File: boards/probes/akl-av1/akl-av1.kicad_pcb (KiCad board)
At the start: 4 copper layers, 23.8 x 10.5 mm, 35 parts, among them J1 U.FL, J2 TIPRES, J3 TIPRES, J4 SMPM, U1 LTC1983-5, U2 ADP7142ACPZN-R7, U3 ADP7182_DFN8, U4 BUF802

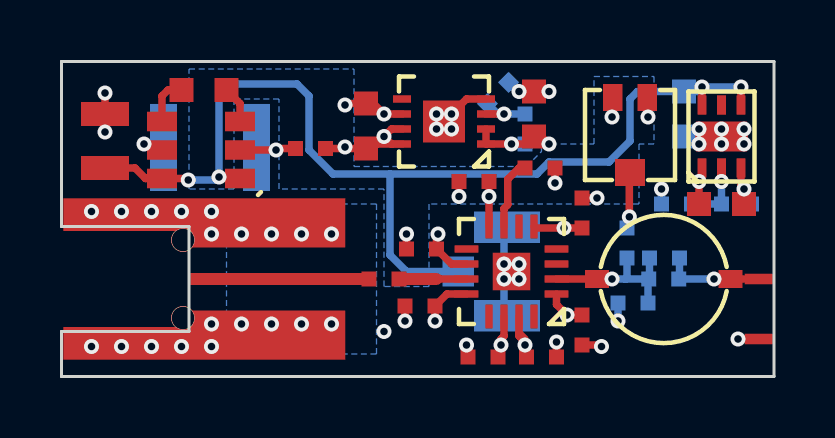
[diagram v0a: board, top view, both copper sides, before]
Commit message: Updated AKL-AV1 design files for v0.3 prototype
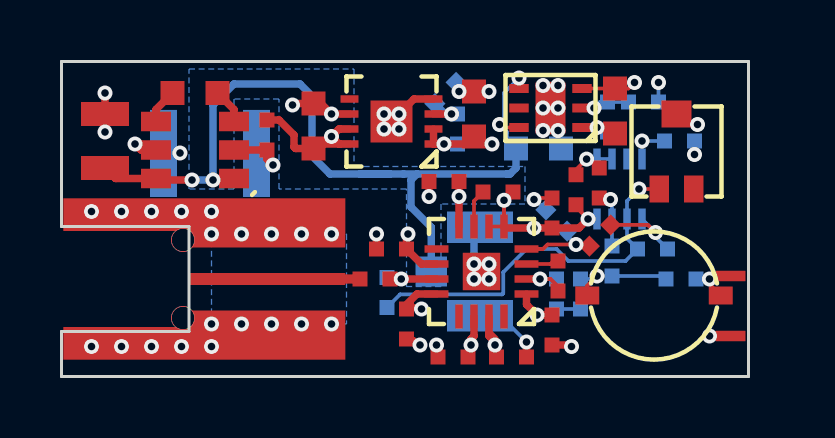
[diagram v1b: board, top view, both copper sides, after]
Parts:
- added C17: 0.47 uF, azonenberg_pcb:EIA_0402_CAP_NOSILK, F.Cu at (64.4, 48.0)
- added C18: 56 pF, azonenberg_pcb:EIA_0402_CAP_NOSILK, B.Cu at (67.0, 50.0)
- added C19: 330 pF, azonenberg_pcb:EIA_0402_CAP_NOSILK, B.Cu at (63.8, 51.5)
- added C20: 100 pF, azonenberg_pcb:EIA_0402_CAP_NOSILK, B.Cu at (63.8, 49.0)
- added R12: 80.6K, azonenberg_pcb:EIA_0402_RES_NOSILK, B.Cu at (58.1, 51.5)
- added R13: 2K, azonenberg_pcb:EIA_0402_RES_NOSILK, F.Cu at (65.2, 49.5)
- added R14: 10M, azonenberg_pcb:EIA_0402_RES_NOSILK, F.Cu at (63.8, 50.9)
- added R9: 3312J-1-203E, azonenberg_pcb:RES_TRIM_BOURNS_3312, F.Cu at (67.8, 46.8)
- added U5: ADA4075-2, azonenberg_pcb:DFN_8_0.5MM_2x2MM_NOPAD, B.Cu at (65.8, 48.0)
- C16: value 800 fF -> 0.47 uF
- R11: value 3312J-1-103E1 -> 30; footprint azonenberg_pcb:RES_TRIM_BOURNS_3312 -> azonenberg_pcb:EIA_0402_RES_NOSILK; moved to B.Cu
- R6: value 1M -> 806K
- R7: value 1M -> 200K; footprint azonenberg_pcb:EIA_0402_CAP_NOSILK -> azonenberg_pcb:EIA_0402_RES_NOSILK; moved to F.Cu
- moved U2 5.78 mm to (63.5, 45.3), turned to 90 degrees
- moved R11 5.55 mm to (64.5, 51.5), turned to -90 degrees
- moved C3 4.98 mm to (63.1, 46.6), turned to 180 degrees
- moved C6 4.71 mm to (65.7, 45.4), turned to -90 degrees
- moved R4 4.60 mm to (66.7, 45.1)
- moved C16 3.93 mm to (67.8, 46.4), turned to 0 degrees
- moved R3 3.70 mm to (65.5, 45.6), turned to 90 degrees
- moved R1 2.25 mm to (60.5, 46.0)
- moved R7 2.20 mm to (65.2, 47.8)
- moved C4 2.00 mm to (61.0, 45.5)
- moved C2 1.75 mm to (55.6, 45.9)
- moved R2 1.75 mm to (60.0, 44.8)
- moved U3 1.75 mm to (58.2, 45.8)
- moved R8 1.61 mm to (61.8, 48.1)
- moved R6 1.57 mm to (65.6, 50.4), turned to 90 degrees
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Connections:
- C16 pad 1: /TIP -> /4V5_P
- C16 pad 2: /VIN -> /GND
- L1 pad 1: Net-(C7-Pad1) -> /Power Supply/5V0_N
- L1 pad 2: /Power Supply/5V0_N -> Net-(C7-Pad1)
- R11 pad 1: /4V5_P -> /VIN
- R11 pad 2: Net-(R11-Pad2) -> Net-(C19-Pad1)
- R6 pad 2: /GND -> Net-(R6-Pad2)
- R7 pad 1: /VIN -> Net-(R6-Pad2)
- R7 pad 2: Net-(R11-Pad2) -> /GND
- U4 pad 2: /VIN -> Net-(U4-Pad2)
- U4 pad 3: unconnected-(U4-Pad3) -> Net-(U4-Pad3)
- U4 pad 4: unconnected-(U4-Pad4) -> /VAUX
- U4 pad 6: unconnected-(U4-Pad6) -> /4V5_N
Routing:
- net Net-(R9-Pad1): track 0.00 -> 12.9 mm, vias 0 -> 1
- net /Power Supply/6V0: track 35.7 -> 29.0 mm
- net Net-(R13-Pad1): track 0.00 -> 2.95 mm, vias 0 -> 1
- net /GND: track 81.8 -> 84.4 mm, vias 48 -> 51
- net /4V5_N: track 25.7 -> 28.2 mm
- net /VAUX: track 0.00 -> 2.13 mm, vias 0 -> 1
- net Net-(R11-Pad2): track 1.89 -> 0.00 mm, vias 1 -> 0
- net Net-(R6-Pad2): track 0.00 -> 1.71 mm, vias 0 -> 1
- net /VIN: track 5.28 -> 3.58 mm
- net Net-(U4-Pad2): track 0.00 -> 1.70 mm, vias 0 -> 1
- net /TIP: track 3.41 -> 1.90 mm
- net Net-(U4-Pad3): track 0.00 -> 1.15 mm
- net /RBIAS: track 2.36 -> 1.27 mm
- net Net-(R12-Pad2): track 2.25 -> 1.17 mm, vias 0 -> 1
- net Net-(C19-Pad1): track 0.00 -> 0.80 mm
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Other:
- board size 23.8 x 10.5 mm -> 22.9 x 10.5 mm
- board text added: "2022-07-03 A. Zonenberg"
- board text added: "AKL-AV1 v0.3"
- board text removed: "AKL-AV1 v0.2 2022-06-21 A. Zonenberg"
